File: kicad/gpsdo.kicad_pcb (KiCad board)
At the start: 4 copper layers, 101.6 x 76.2 mm, 18 parts, among them J1 Conn_Coaxial, J2 Conn_01x04_Male, J3 Conn_01x04_Male, J4 Conn_01x04_Male, J5 Conn_01x04_Male, U1 MSP430F5171IDA, U2 MAX-8Q, U3 549CAAC000111BBG, U4 Si7051-A20

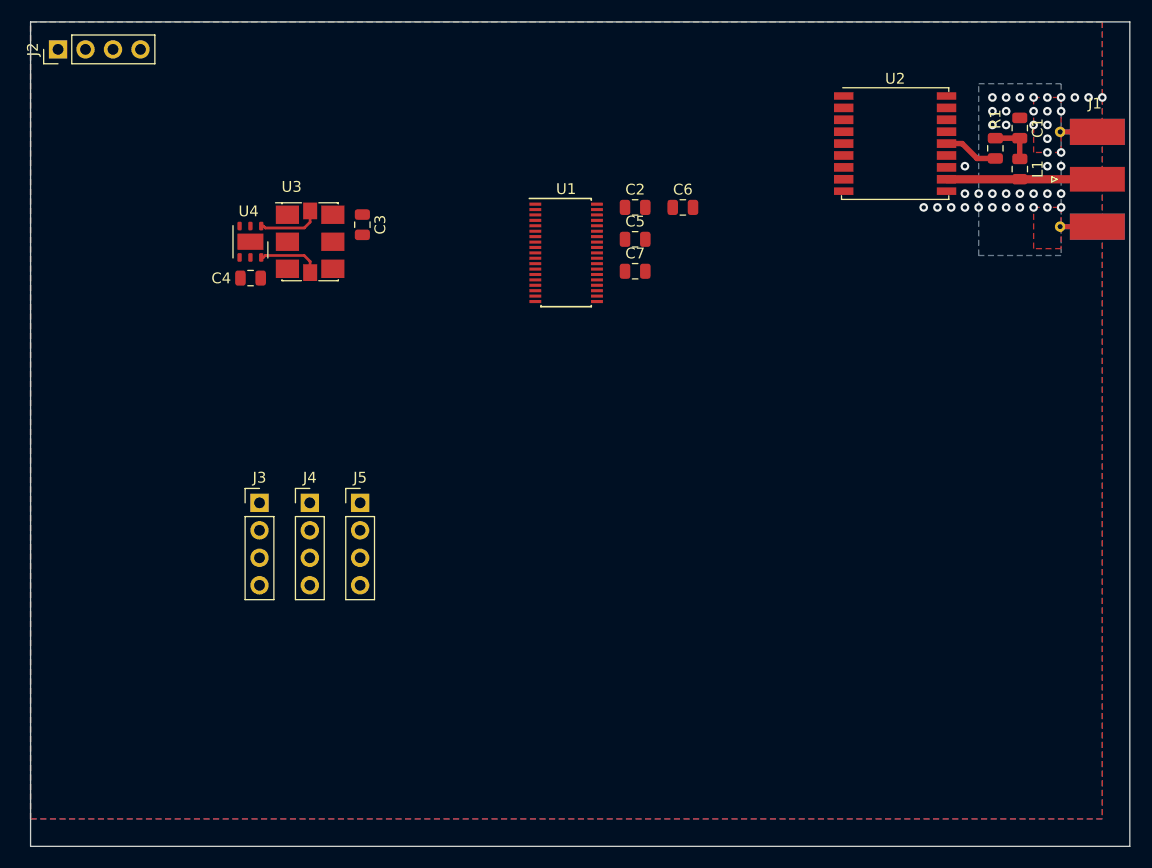
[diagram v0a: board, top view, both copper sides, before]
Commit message: update board layout
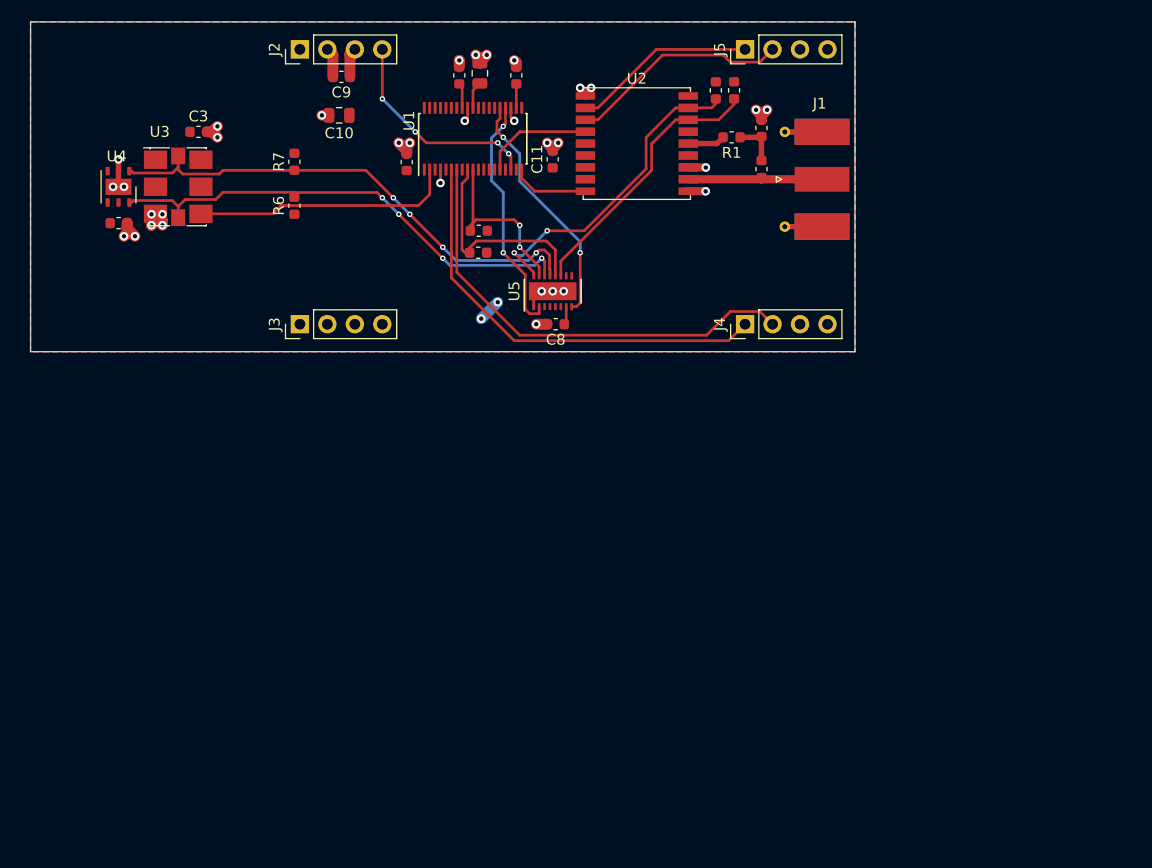
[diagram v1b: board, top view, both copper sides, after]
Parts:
- added C10: 10u, Capacitor_SMD:C_0805_2012Metric, F.Cu at (53.9, 34.0)
- added C11: 100n, Resistor_SMD:R_0603_1608Metric, F.Cu at (73.7, 38.1)
- added C8: 100n, Resistor_SMD:R_0603_1608Metric, F.Cu at (73.9, 53.3)
- added C9: 100n, Resistor_SMD:R_0603_1608Metric, F.Cu at (54.1, 30.5)
- added R2: 1.5k, Resistor_SMD:R_0603_1608Metric, F.Cu at (66.8, 44.7)
- added R3: 1.5k, Resistor_SMD:R_0603_1608Metric, F.Cu at (66.8, 46.7)
- added R4: 1.5k, Resistor_SMD:R_0603_1608Metric, F.Cu at (88.7, 31.7)
- added R5: 1.5k, Resistor_SMD:R_0603_1608Metric, F.Cu at (90.4, 31.7)
- added R6: 1.5k, Resistor_SMD:R_0603_1608Metric, F.Cu at (49.8, 42.4)
- added R7: 1.5k, Resistor_SMD:R_0603_1608Metric, F.Cu at (49.8, 38.3)
- added U5: LTC4317, Package_DFN_QFN:DFN-16-1EP_3x5mm_P0.5mm_EP1.66x4.4mm, F.Cu at (73.7, 50.3)
- C1, C2, C3, C4, C5, C6: footprint Capacitor_SMD:C_0805_2012Metric -> Resistor_SMD:R_0603_1608Metric
- L1: footprint Inductor_SMD:L_0805_2012Metric -> Resistor_SMD:R_0603_1608Metric
- R1: footprint Resistor_SMD:R_0805_2012Metric -> Resistor_SMD:R_0603_1608Metric
- moved J5 55.0 mm to (91.4, 27.9), turned to 90 degrees
- moved J4 43.5 mm to (91.4, 53.3), turned to 90 degrees
- moved C6 25.9 mm to (60.2, 38.3), turned to 90 degrees
- moved J1 25.4 mm to (96.8, 39.9)
- moved R1 24.4 mm to (90.2, 36.1), turned to 180 degrees
- moved L1 23.9 mm to (93.0, 39.0)
- moved U2 23.9 mm to (81.4, 36.6)
- moved C1 23.9 mm to (93.0, 35.2)
- moved C7 23.3 mm to (66.9, 30.1), turned to 90 degrees
- moved J2 22.4 mm to (50.3, 27.9)
- moved C2 20.3 mm to (65.0, 30.3), turned to 90 degrees
- moved C5 18.7 mm to (70.3, 30.3), turned to 90 degrees
- moved C3 17.4 mm to (40.9, 35.6), turned to 0 degrees
- moved J3 16.9 mm to (50.3, 53.3), turned to 90 degrees
- moved U1 13.6 mm to (66.3, 36.2), turned to 90 degrees
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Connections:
- net Net-(U1-Pad16) renamed oPPS
- J2 pad 3: GND -> +3V3
- J2 pad 4: GND -> ePPS
- J4 pad 1: GND -> Net-(J4-Pad1)
- J4 pad 2: GND -> Net-(J4-Pad2)
- J5 pad 1: GND -> Net-(J5-Pad1)
- J5 pad 2: GND -> Net-(J5-Pad2)
- U1 pad 17: Net-(U1-Pad17) -> ePPS
- U1 pad 6: Net-(U1-Pad6) -> Net-(J4-Pad1)
- U1 pad 7: Net-(U1-Pad7) -> Net-(J4-Pad2)
- U2 pad 16: Net-(U2-Pad16) -> Net-(R5-Pad1)
- U2 pad 17: Net-(U2-Pad17) -> Net-(R4-Pad2)
- U2 pad 2: Net-(U2-Pad2) -> Net-(J5-Pad1)
- U2 pad 3: Net-(U2-Pad3) -> Net-(J5-Pad2)
- U2 pad 9: Net-(U2-Pad9) -> Net-(U1-Pad19)
- U3 pad 1: Net-(U3-Pad1) -> +3V3
- U3 pad 7: Net-(U2-Pad16) -> Net-(R7-Pad1)
- U3 pad 8: Net-(U2-Pad17) -> Net-(R6-Pad2)
- U4 pad 1: Net-(U2-Pad16) -> Net-(R7-Pad1)
- U4 pad 4: Net-(U4-Pad4) -> +3V3
- U4 pad 6: Net-(U2-Pad17) -> Net-(R6-Pad2)
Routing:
- net Net-(R7-Pad1): track 0.00 -> 46.7 mm, vias 0 -> 4
- net Net-(R6-Pad2): track 0.00 -> 45.2 mm, vias 0 -> 4
- net Net-(J4-Pad2): track 0.00 -> 42.5 mm
- net Net-(J4-Pad1): track 0.00 -> 40.2 mm
- net GND: track 0.00 -> 36.5 mm, vias 43 -> 33
- net Net-(R4-Pad2): track 0.00 -> 29.6 mm, vias 0 -> 2
- net Net-(R5-Pad1): track 0.00 -> 25.3 mm
- net CLK_25M: track 0.00 -> 24.2 mm
- net Net-(U1-Pad23): track 0.00 -> 22.5 mm, vias 0 -> 2
- net Net-(U1-Pad24): track 0.00 -> 22.3 mm, vias 0 -> 2
- net Net-(J5-Pad2): track 0.00 -> 20.5 mm
- net ePPS: track 0.00 -> 19.9 mm, vias 0 -> 4
- net Net-(R3-Pad1): track 0.00 -> 19.8 mm
- net Net-(J5-Pad1): track 0.00 -> 17.0 mm
- net Net-(R2-Pad2): track 0.00 -> 16.7 mm, vias 0 -> 2
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- added copper zone on F.Cu, net +3V3
- removed copper zone on F.Cu, net GND
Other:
- board size 101.6 x 76.2 mm -> 76.2 x 30.5 mm
- copper layers 4 -> 2
